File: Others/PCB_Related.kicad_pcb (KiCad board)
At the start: 4 copper layers, 70.5 x 43.5 mm, 9 parts, among them U4 MOUDLE-SEEEDUINO-XIAO

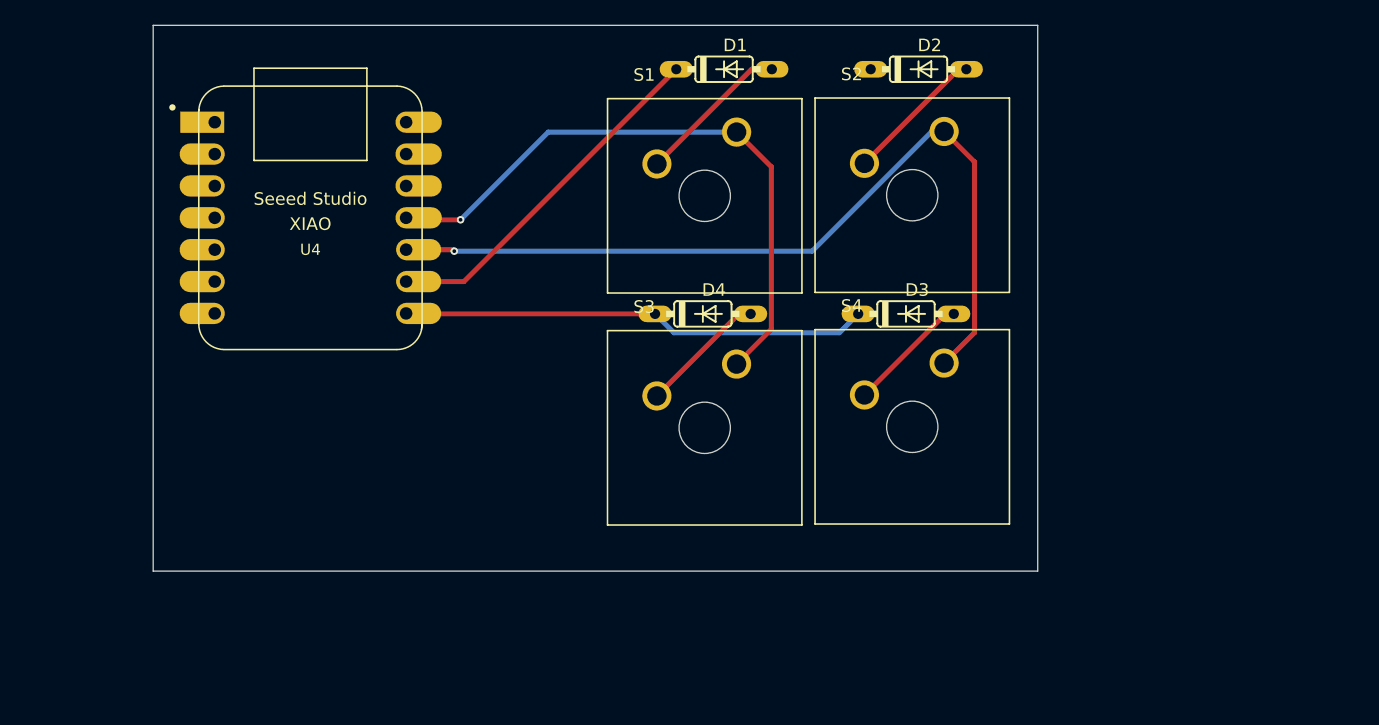
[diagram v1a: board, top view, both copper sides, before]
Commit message: Added pictures and finished cad
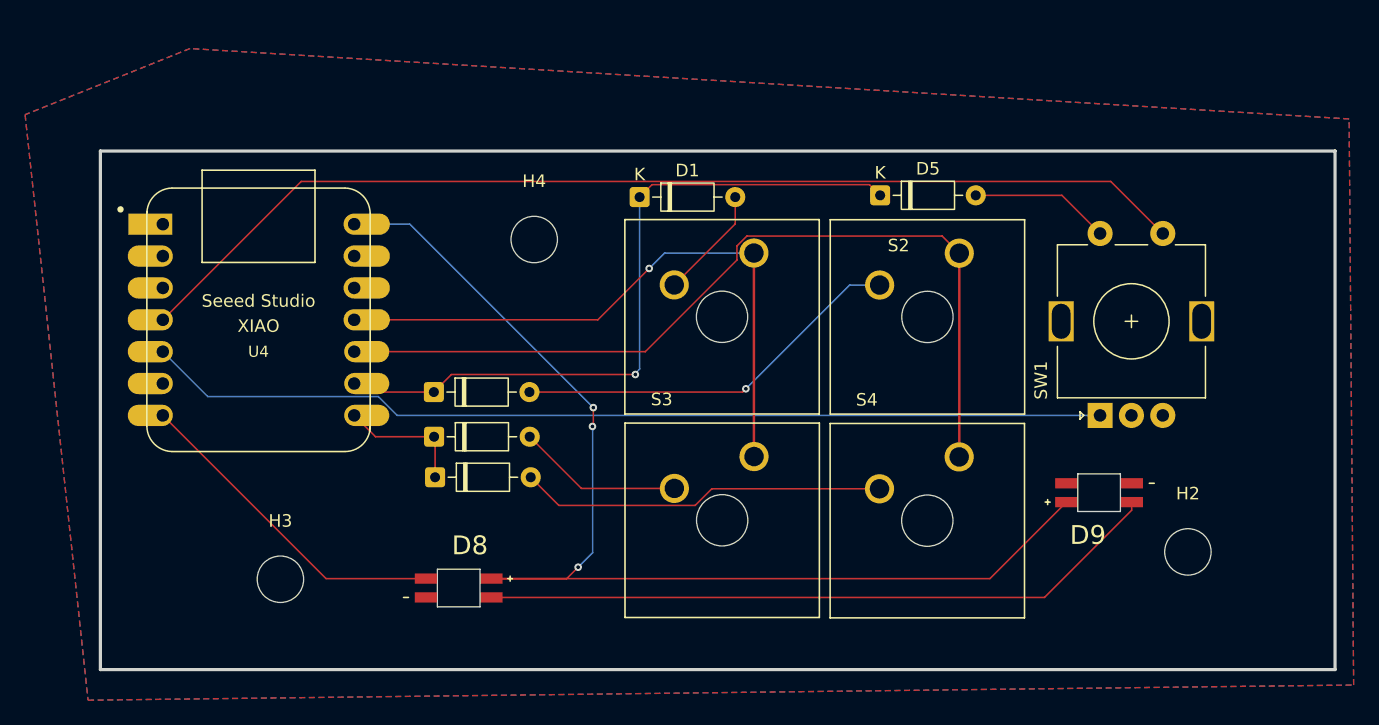
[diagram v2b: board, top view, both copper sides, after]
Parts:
- added D5: D_Small, Diode_THT:D_DO-35_SOD27_P7.62mm_Horizontal, F.Cu at (121.9, 31.1)
- added D8: SK6812-E, SK6812-E:LED_SK6812-E, F.Cu at (88.3, 62.4)
- added D9: SK6812-E, SK6812-E:LED_SK6812-E, F.Cu at (139.4, 54.8)
- added H2: MountingHole, MountingHole:MountingHole_3.7mm, F.Cu at (146.5, 59.5)
- added H3: MountingHole, MountingHole:MountingHole_3.7mm, F.Cu at (74.1, 61.6)
- added H4: MountingHole, MountingHole:MountingHole_3.7mm, F.Cu at (94.4, 34.6)
- added SW1: RotaryEncoder_Switch, Rotary_Encoder:RotaryEncoder_Alps_EC11E-Switch_Vertical_H20mm, F.Cu at (139.5, 48.6)
- D1, D2, D3, D4: value 1N4148 -> D_Small; footprint 1N4148:DO35-7 -> Diode_THT:D_DO-35_SOD27_P7.62mm_Horizontal
- moved D2 46.4 mm to (86.4, 46.7)
- moved D3 38.9 mm to (86.4, 50.3)
- moved D4 25.0 mm to (86.5, 53.5)
- moved D1 12.2 mm to (102.8, 31.2)
- moved S2 9.78 mm to (125.7, 40.7)
- moved S1 9.74 mm to (109.3, 40.7)
- moved U4 9.12 mm to (72.4, 41.0)
- moved S4 7.58 mm to (125.7, 57.0)
- moved S3 7.50 mm to (109.3, 57.0)
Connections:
- S1 pad 1: Net-(D1-PadA) -> Net-(D1-A)
- S2 pad 1: Net-(D2-PadA) -> Net-(D2-A)
- S3 pad 1: Net-(D4-PadA) -> Net-(D3-A)
- S4 pad 1: Net-(D3-PadA) -> Net-(D4-A)
- U4 pad 14: unconnected-(U4-5V-Pad14) -> VCC
- U4 pad 4: unconnected-(U4-PA11_A3_D3-Pad4) -> B
- U4 pad 5: unconnected-(U4-PA8_A4_D4_SDA-Pad5) -> AUP
- U4 pad 6: unconnected-(U4-PA9_A5_D5_SCL-Pad6) -> BDOWN
- U4 pad 7: unconnected-(U4-PB08_A6_D6_TX-Pad7) -> LED
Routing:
- net VCC: track 0.00 -> 94.0 mm, vias 0 -> 3
- net B: track 0.00 -> 86.0 mm
- net AUP: track 0.00 -> 76.8 mm
- net Net-(D8-DOUT): track 0.00 -> 54.6 mm
- net Net-(D2-A): track 0.00 -> 31.4 mm, vias 0 -> 1
- net ROW0: track 28.1 -> 57.5 mm, vias 0 -> 1
- net Net-(D4-A): track 0.00 -> 29.3 mm
- net ROW1: track 36.8 -> 10.3 mm
- net LED: track 0.00 -> 26.4 mm
- net Net-(D3-A): track 0.00 -> 13.2 mm
- net Net-(D1-PadA): track 12.3 -> 0.00 mm
- net Net-(D2-PadA): track 11.2 -> 0.00 mm
- net A: track 0.00 -> 11.2 mm
- net Net-(D4-PadA): track 10.2 -> 0.00 mm
- net Net-(D3-PadA): track 9.80 -> 0.00 mm
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- added copper zone on B.Cu, net GND
- added copper zone on F.Cu, net GND
- added copper zone on In1.Cu, net GND
- added copper zone on In2.Cu, net GND
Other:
- board size 70.5 x 43.5 mm -> 98.4 x 41.3 mm
